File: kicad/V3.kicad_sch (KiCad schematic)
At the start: 54 parts, among them SW1 KS33_SW_HS, SW10 KS33_SW_HS, SW11 KS33_SW_HS, SW12 KS33_SW_HS, SW13 KS33_SW_HS, SW14 KS33_SW_HS, SW15 KS33_SW_HS, SW16 KS33_SW_HS, SW17 KS33_SW_HS, SW18 KS33_SW_HS, SW19 KS33_SW_HS, SW2 KS33_SW_HS, SW20 KS33_SW_HS, SW21 KS33_SW_HS, SW22 KS33_SW_HS, SW23 KS33_SW_HS, SW3 KS33_SW_HS, SW4 KS33_SW_HS, SW5 KS33_SW_HS, SW6 KS33_SW_HS, SW7 KS33_SW_HS, SW8 KS33_SW_HS, SW9 KS33_SW_HS, U4 SSD1306-128X64-OLED-0.96

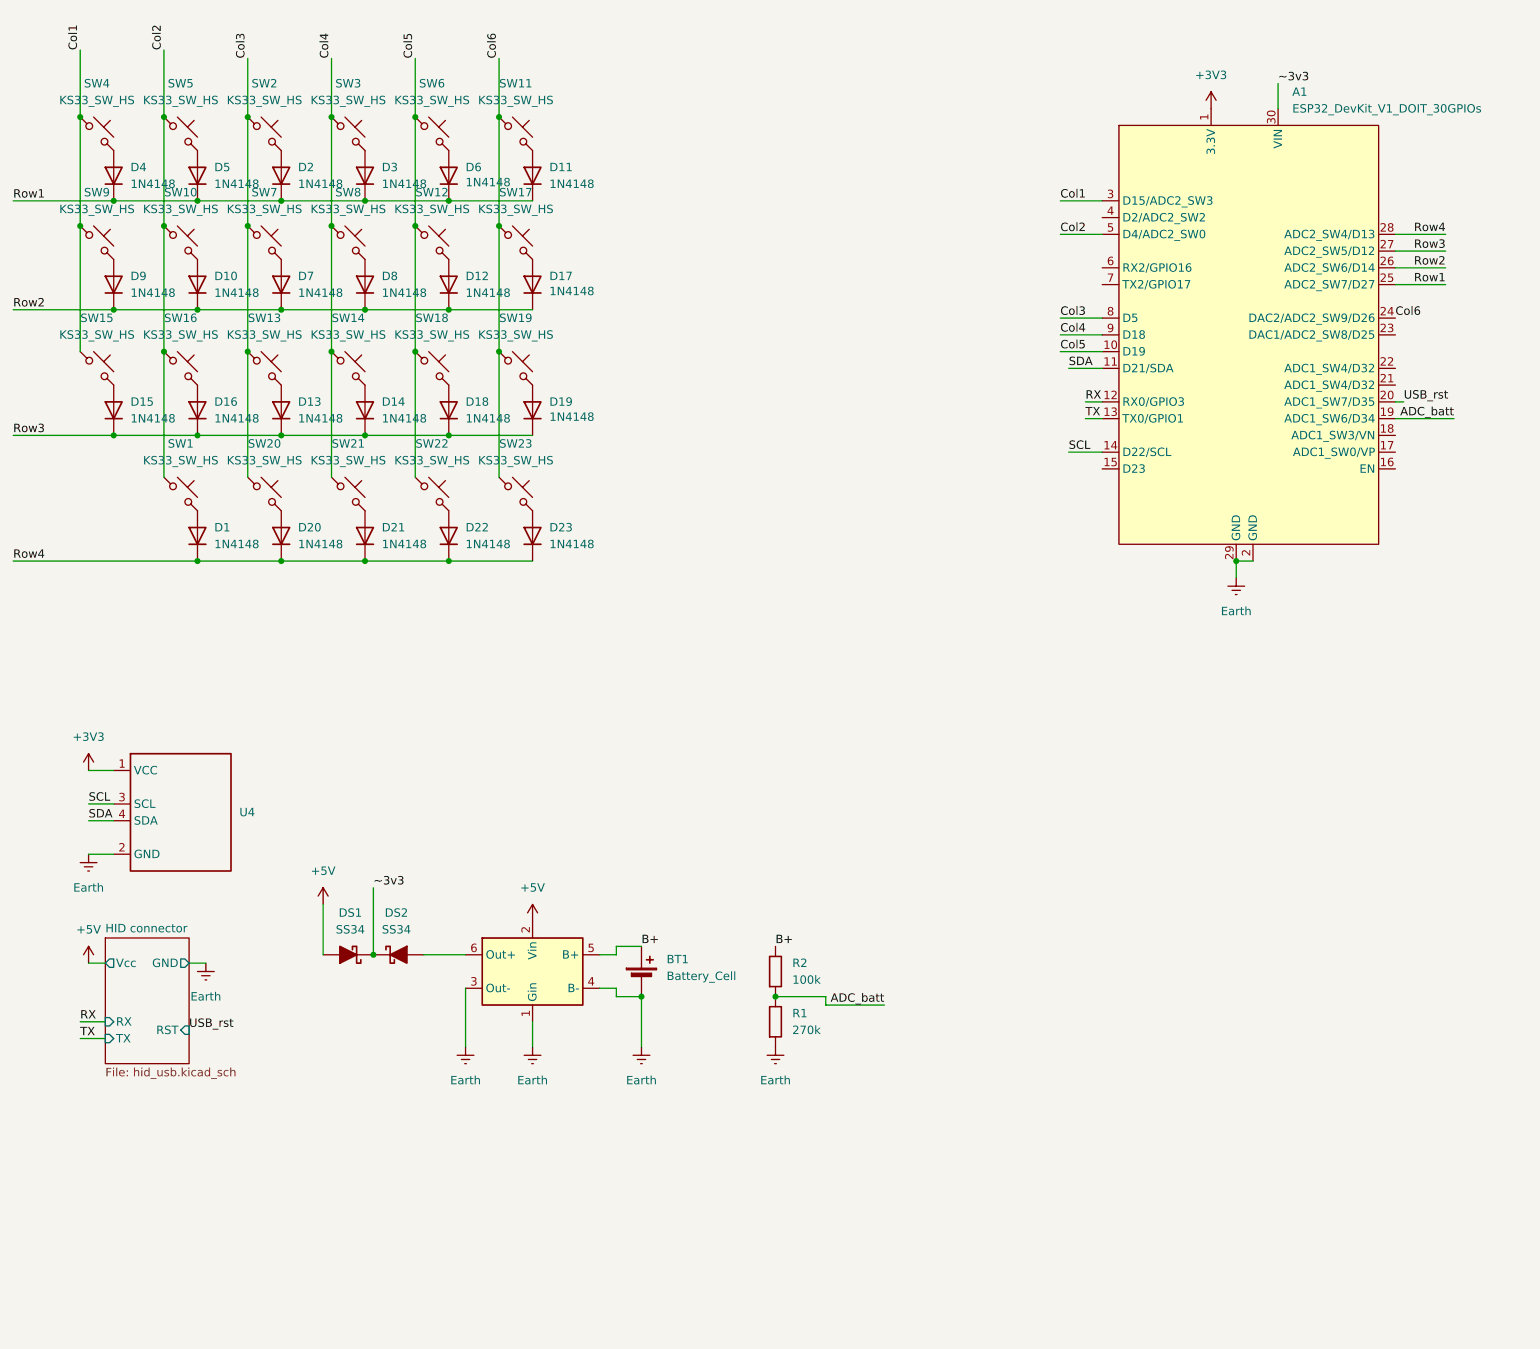
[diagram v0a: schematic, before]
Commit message: working version
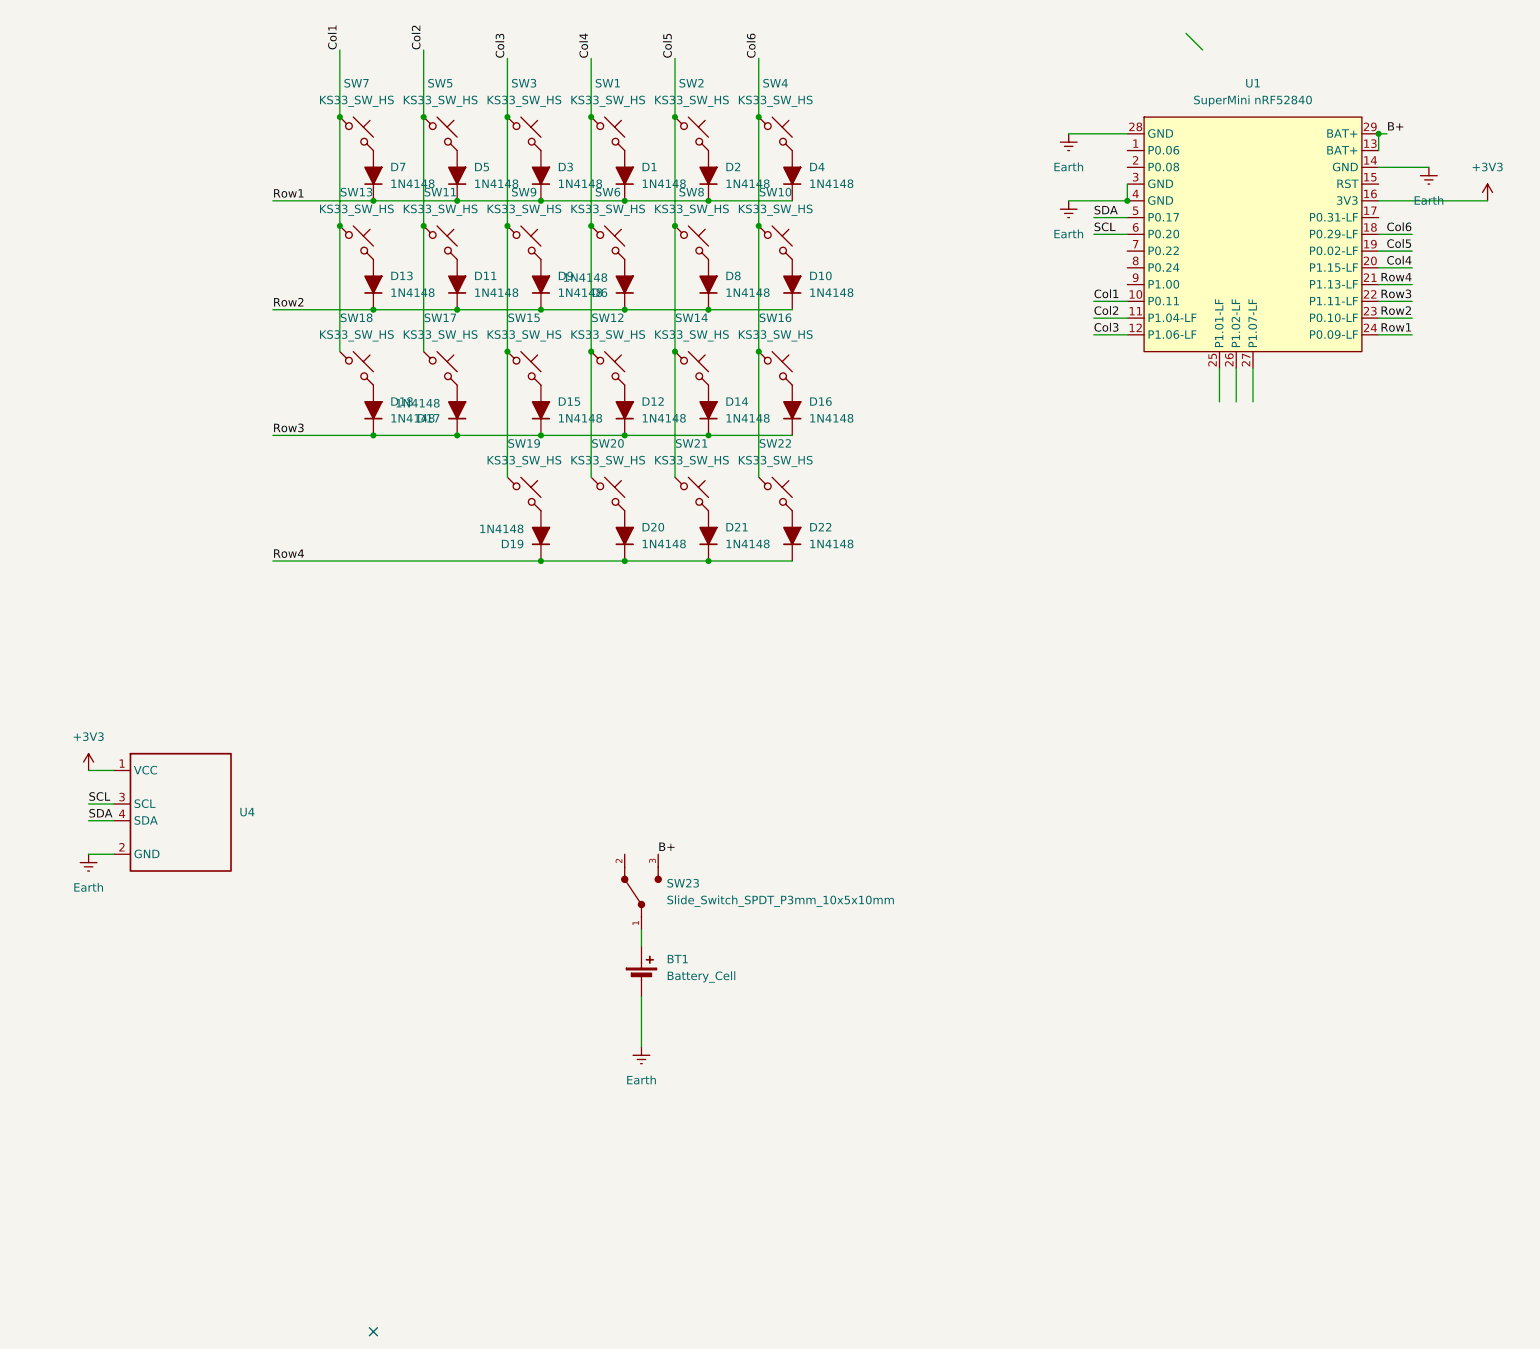
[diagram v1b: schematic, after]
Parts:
- removed A1: ESP32_DevKit_V1_DOIT_30GPIOs, PCM_SL_Development_Boards:DOIT_ESP32_DEVKIT_30Pins, symbol PCM_SL_Development_Board:ESP32_DevKit_V1_DOIT_30GPIOs
- removed D22, D23: 1N4148, Diode_THT:D_DO-35_SOD27_P7.62mm_Horizontal, symbol Diode:1N4148
- removed DS1, DS2: SS34, PCM_Diode_SMD_AKL:D_SMC, symbol PCM_Diode_Schottky_AKL:SS34
- removed R1: 270k, Resistor_THT:R_Axial_DIN0207_L6.3mm_D2.5mm_P10.16mm_Horizontal, symbol PCM_SL_Resistors:270k
- removed R2: 100k, Resistor_THT:R_Axial_DIN0207_L6.3mm_D2.5mm_P10.16mm_Horizontal, symbol PCM_SL_Resistors:100k
- removed SW23: KS33_SW_HS, keyswitches:Kailh_socket_MX_reversible, symbol PCM_marbastlib-gateron_lp:KS33_SW_HS_KS-2P02B01-02
- removed U1: ~, Library:HAYATEC TP4056 LIPO SWARGING MODULE, symbol Library:TP4056_usb_module
- added D22: 1N4148, PCM_Diode_THT_AKL:D_DO-35_SOD27_P7.62mm_Horizontal, symbol PCM_Diode_AKL:1N4148
- added SW23: Slide_Switch_SPDT_P3mm_10x5x10mm, PCM_SL_Devices:Slide_Switch_SPDT_P3mm_10x5x10mm, symbol PCM_SL_Devices:Slide_Switch_SPDT_P3mm_10x5x10mm
- added U1: SuperMini nRF52840, PCM_marbastlib-xp-promicroish:SuperMini_nRF52840_AH_USBup, symbol PCM_marbastlib-promicroish:SuperMini_nRF52840
- D1, D10, D11, D12, D13, D14, D15, D16, D17, D18, D19, D2, D20, D21, D3, D4, D5, D6, D7, D8, D9: footprint Diode_THT:D_DO-35_SOD27_P7.62mm_Horizontal -> PCM_Diode_THT_AKL:D_DO-35_SOD27_P7.62mm_Horizontal; symbol Diode:1N4148 -> PCM_Diode_AKL:1N4148
- SW1, SW10, SW11, SW12, SW13, SW14, SW15, SW16, SW17, SW18, SW19, SW2, SW20, SW21, SW22, SW3, SW4, SW5, SW6, SW7, SW8, SW9: footprint keyswitches:Kailh_socket_MX_reversible -> keyswitches:Kailh_socket_PG1350_reversible
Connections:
- net +3V3: now also U1.16 (3V3)
- net B+: now also SW23.3, U1.13 (BAT+), U1.29 (BAT+); no longer BT1.1 (+)
- net Col1: now also SW13.1, SW18.1, SW7.1, U1.10 (P0.11); no longer SW15.1, SW4.1, SW9.1
- net Col2: now also SW11.1, SW17.1, U1.11 (P1.04-LF); no longer SW1.1, SW10.1, SW16.1
- net Col3: now also SW15.1, SW19.1, SW3.1, SW9.1, U1.12 (P1.06-LF); no longer SW13.1, SW2.1, SW20.1, SW7.1
- net Col4: now also SW1.1, SW12.1, SW20.1, SW6.1, U1.20 (P1.15-LF); no longer SW14.1, SW21.1, SW3.1, SW8.1
- net Col5: now also SW14.1, SW2.1, SW21.1, SW8.1, U1.19 (P0.02-LF); no longer SW12.1, SW18.1, SW22.1, SW6.1
- net Col6: now also SW10.1, SW16.1, SW22.1, SW4.1, U1.18 (P0.29-LF); no longer SW11.1, SW17.1, SW19.1
- net Earth: now also U1.14 (GND), U1.28 (GND), U1.3 (GND), U1.4 (GND)
- net Row1: now also D1.1 (K), D7.1 (K), U1.24 (P0.09-LF); no longer D11.1 (K), D6.1 (K)
- net Row2: now also D11.1 (K), D13.1 (K), D6.1 (K), U1.23 (P0.10-LF); no longer D12.1 (K), D17.1 (K), D7.1 (K)
- net Row3: now also D12.1 (K), D17.1 (K), U1.22 (P1.11-LF); no longer D13.1 (K), D19.1 (K)
- net Row4: now also D19.1 (K), D22.1 (K), U1.21 (P1.13-LF); no longer D1.1 (K)
- net SCL: now also U1.6 (P0.20)
- net SDA: now also U1.5 (P0.17)
- net at SW22.2: now also D22.2 (A)
- new net: BT1.1 (+), SW23.1
- no-connect marks 0 -> 1
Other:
- removed sheet HID connector
- moved on the sheet: SW1, SW10, SW11, SW12, SW13, SW14, SW15, SW16, SW17, SW18, SW19, SW2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
